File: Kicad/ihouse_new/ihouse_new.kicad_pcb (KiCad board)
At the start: 2 copper layers, 51 parts, among them U1 PCF8583T, U10 MOC3063M, U11 MOC3063M, U12 MOC3063M, U2 MCP23017-E_SO, U3 L293D, U4 L293D, U5 MOC3063M, U6 MOC3063M, U7 MOC3063M, U8 MOC3063M, U9 MOC3063M, Y1 32768

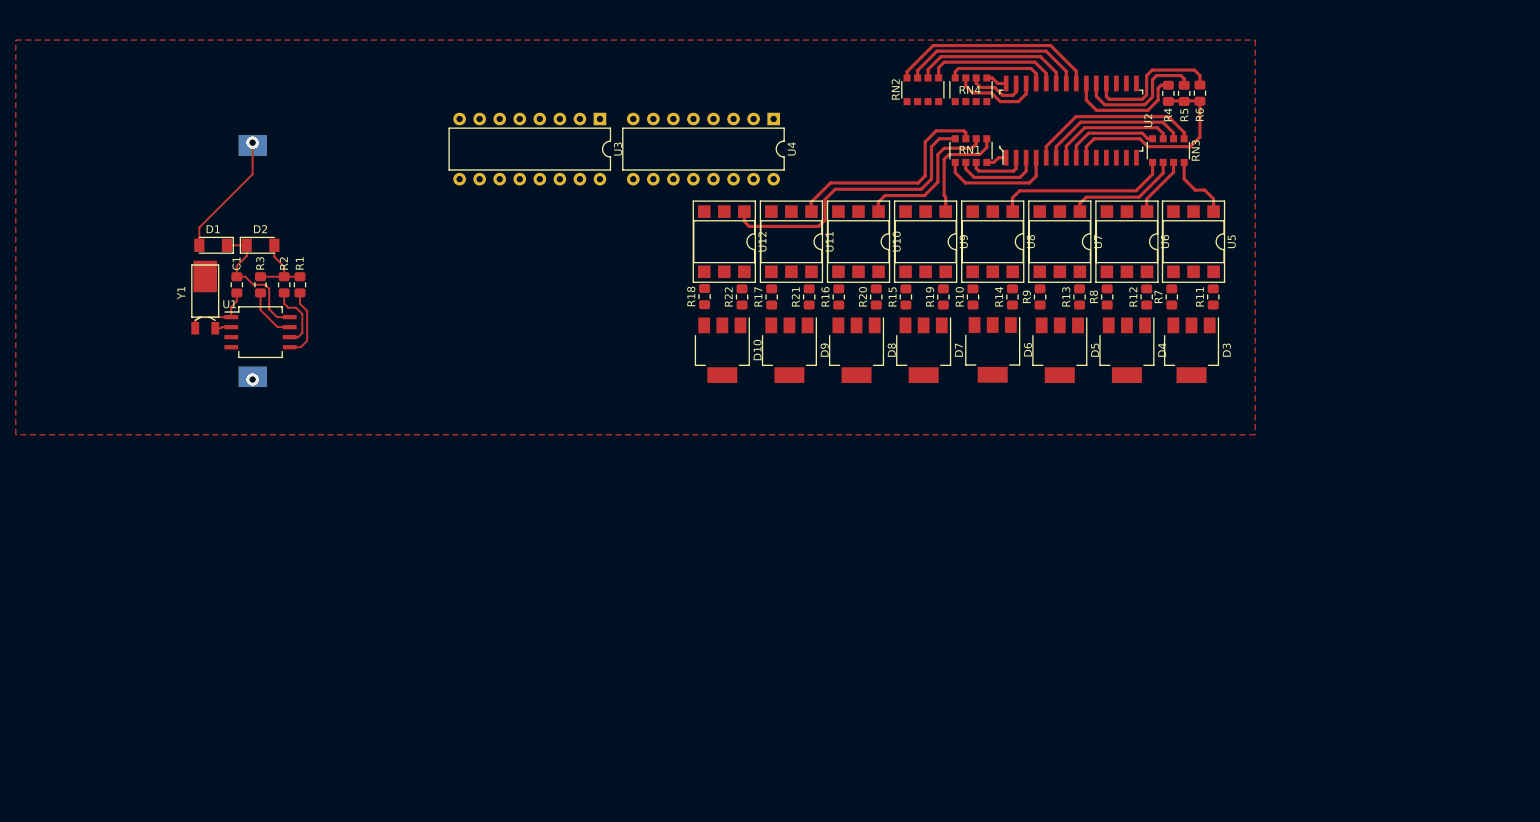
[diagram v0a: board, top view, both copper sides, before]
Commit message: schemos paruosimas
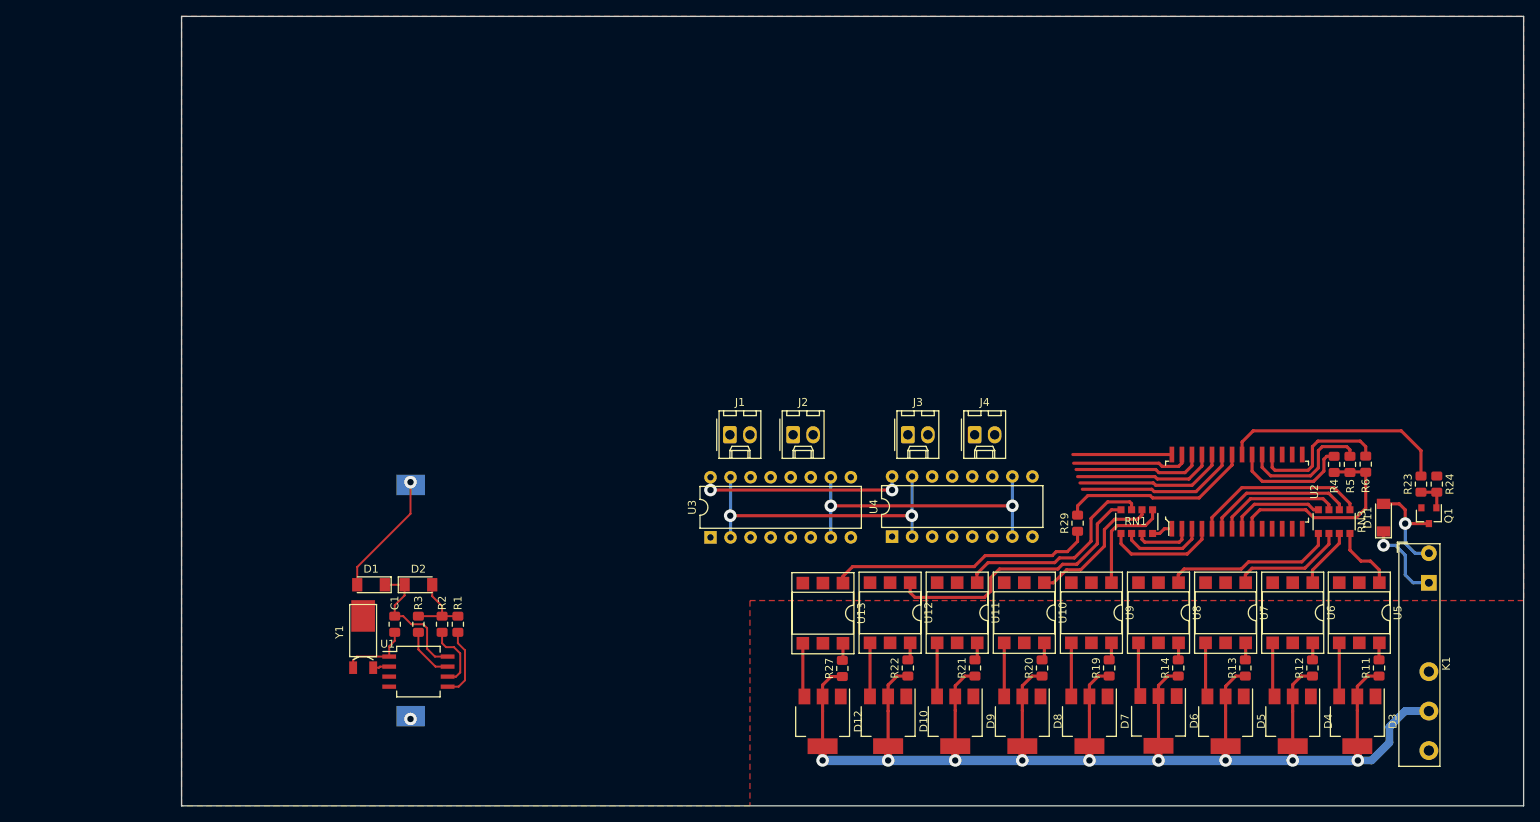
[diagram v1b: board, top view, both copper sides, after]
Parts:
- removed R10, R15, R16, R17, R18, R7, R8, R9: 300, Resistor_SMD:R_0805_2012Metric_Pad1.15x1.40mm_HandSolder
- removed RN2, RN4: R_Pack04, Resistor_SMD:R_Array_Convex_4x1206
- added D11: BAS32, Diode_SMD:D_MiniMELF, F.Cu at (216.2, 95.5)
- added D12: Z0103MN, Package_TO_SOT_SMD:SOT-223, F.Cu at (145.2, 121.3)
- added J1: Valve 1, Connector_Molex:Molex_KK-254_AE-6410-02A_1x02_P2.54mm_Vertical, F.Cu at (133.5, 85.0)
- added J2: Valve 1, Connector_Molex:Molex_KK-254_AE-6410-02A_1x02_P2.54mm_Vertical, F.Cu at (141.5, 85.0)
- added J3: Valve 1, Connector_Molex:Molex_KK-254_AE-6410-02A_1x02_P2.54mm_Vertical, F.Cu at (156.0, 85.0)
- added J4: Valve 1, Connector_Molex:Molex_KK-254_AE-6410-02A_1x02_P2.54mm_Vertical, F.Cu at (164.5, 85.0)
- added K1: FINDER-32.21-x000, Relay_THT:Relay_SPDT_Finder_34.51_Vertical, F.Cu at (222.0, 103.8)
- added Q1: BC817, Package_TO_SOT_SMD:SOT-23, F.Cu at (222.0, 95.2)
- added R23: 10k, Resistor_SMD:R_0805_2012Metric_Pad1.15x1.40mm_HandSolder, F.Cu at (221.0, 91.2)
- added R24: 1k, Resistor_SMD:R_0805_2012Metric_Pad1.15x1.40mm_HandSolder, F.Cu at (223.0, 91.2)
- added R27: 470, Resistor_SMD:R_0805_2012Metric_Pad1.15x1.40mm_HandSolder, F.Cu at (147.7, 114.6)
- added R29: 470, Resistor_SMD:R_0805_2012Metric_Pad1.15x1.40mm_HandSolder, F.Cu at (177.5, 96.2)
- added U13: MOC3063M, Package_DIP:DIP-6_W7.62mm_SMDSocket_SmallPads, F.Cu at (145.2, 107.6)
- D1: value BAS32 -> BAS85
- moved U4 55.0 mm to (154.0, 97.9), turned to 90 degrees
- moved U3 54.8 mm to (131.0, 98.0), turned to 90 degrees
- moved D10 51.5 mm to (153.5, 121.3)
- moved D3 51.5 mm to (212.9, 121.3)
- moved D4 51.5 mm to (204.8, 121.3)
- moved D5 51.5 mm to (196.2, 121.3)
- moved D6 51.5 mm to (187.8, 121.2)
- moved D7 51.5 mm to (179.0, 121.3)
- moved D8 51.5 mm to (170.5, 121.3)
- moved D9 51.5 mm to (162.0, 121.3)
- moved R11 51.5 mm to (215.7, 114.5)
- moved R12 51.5 mm to (207.2, 114.5)
- moved R13 51.5 mm to (198.8, 114.5)
- moved R14 51.5 mm to (190.2, 114.5)
- moved R19 51.5 mm to (181.5, 114.5)
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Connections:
- D10 pad 2: Net-(D10-Pad2) -> /ACL
- D10 pad 4: Net-(D10-Pad2) -> /ACL
- D3 pad 2: Net-(D3-Pad2) -> /ACL
- D3 pad 4: Net-(D3-Pad2) -> /ACL
- D4 pad 2: Net-(D4-Pad2) -> /ACL
- D4 pad 4: Net-(D4-Pad2) -> /ACL
- D5 pad 2: Net-(D5-Pad2) -> /ACL
- D5 pad 4: Net-(D5-Pad2) -> /ACL
- D6 pad 2: Net-(D6-Pad2) -> /ACL
- D6 pad 4: Net-(D6-Pad2) -> /ACL
- D7 pad 2: Net-(D7-Pad2) -> /ACL
- D7 pad 4: Net-(D7-Pad2) -> /ACL
- D8 pad 2: Net-(D8-Pad2) -> /ACL
- D8 pad 4: Net-(D8-Pad2) -> /ACL
- D9 pad 2: Net-(D9-Pad2) -> /ACL
- D9 pad 4: Net-(D9-Pad2) -> /ACL
- R11 pad 1: Net-(D3-Pad2) -> /ACL
- R12 pad 1: Net-(D4-Pad2) -> /ACL
- R13 pad 1: Net-(D5-Pad2) -> /ACL
- R14 pad 1: Net-(D6-Pad2) -> /ACL
- R19 pad 1: Net-(D7-Pad2) -> /ACL
- R20 pad 1: Net-(D8-Pad2) -> /ACL
- R21 pad 1: Net-(D9-Pad2) -> /ACL
- R22 pad 1: Net-(D10-Pad2) -> /ACL
- U10 pad 4: Net-(D8-Pad1) -> Net-(D8-Pad3)
- U11 pad 4: Net-(D9-Pad1) -> Net-(D9-Pad3)
- U12 pad 4: Net-(D10-Pad1) -> Net-(D10-Pad3)
- U2 pad 21: Net-(RN2-Pad4) -> /ACON
- U2 pad 23: Net-(RN2-Pad2) -> /MA
- U2 pad 24: Net-(RN2-Pad1) -> /MB
- U2 pad 25: Net-(RN4-Pad4) -> /M1ENA
- U2 pad 26: Net-(RN4-Pad3) -> /M2ENA
- U2 pad 27: Net-(RN4-Pad2) -> /M3ENA
- U2 pad 28: Net-(RN4-Pad1) -> /M4ENA
- U3 pad 10: /MA -> /MB
- U3 pad 15: /MB -> /MA
- U4 pad 10: /MA -> /MB
- U4 pad 15: /MB -> /MA
- U5 pad 4: Net-(D3-Pad1) -> Net-(D3-Pad3)
- U6 pad 4: Net-(D4-Pad1) -> Net-(D4-Pad3)
- U7 pad 4: Net-(D5-Pad1) -> Net-(D5-Pad3)
- U8 pad 4: Net-(D6-Pad1) -> Net-(D6-Pad3)
- U9 pad 4: Net-(D7-Pad1) -> Net-(D7-Pad3)
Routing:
- net /ACL: track 0.00 -> 193.1 mm, vias 0 -> 9
- net /MA: track 0.00 -> 58.9 mm, vias 0 -> 2
- net /MB: track 0.00 -> 57.5 mm, vias 0 -> 2
- net /OC9: track 0.00 -> 33.4 mm
- net /ACON: track 0.00 -> 29.1 mm
- net Net-(RN2-Pad4): track 26.5 -> 0.00 mm
- net +5V: track 35.0 -> 61.3 mm, vias 0 -> 2
- net Net-(RN2-Pad2): track 20.2 -> 0.00 mm
- net /M1ENA: track 0.00 -> 18.0 mm
- net Net-(RN2-Pad1): track 17.1 -> 0.00 mm
- net /M2ENA: track 0.00 -> 16.6 mm
- net /M3ENA: track 0.00 -> 15.1 mm
- net Net-(D11-Pad2): track 0.00 -> 13.8 mm, vias 0 -> 1
- net Net-(RN4-Pad4): track 12.7 -> 0.00 mm
- net /M4ENA: track 0.00 -> 12.5 mm
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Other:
- board outline added: 170 x 100 mm
